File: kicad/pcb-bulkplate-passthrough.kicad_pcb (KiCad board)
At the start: 2 copper layers, 60.8 x 64.2 mm, 9 parts, among them J1 2601-3108

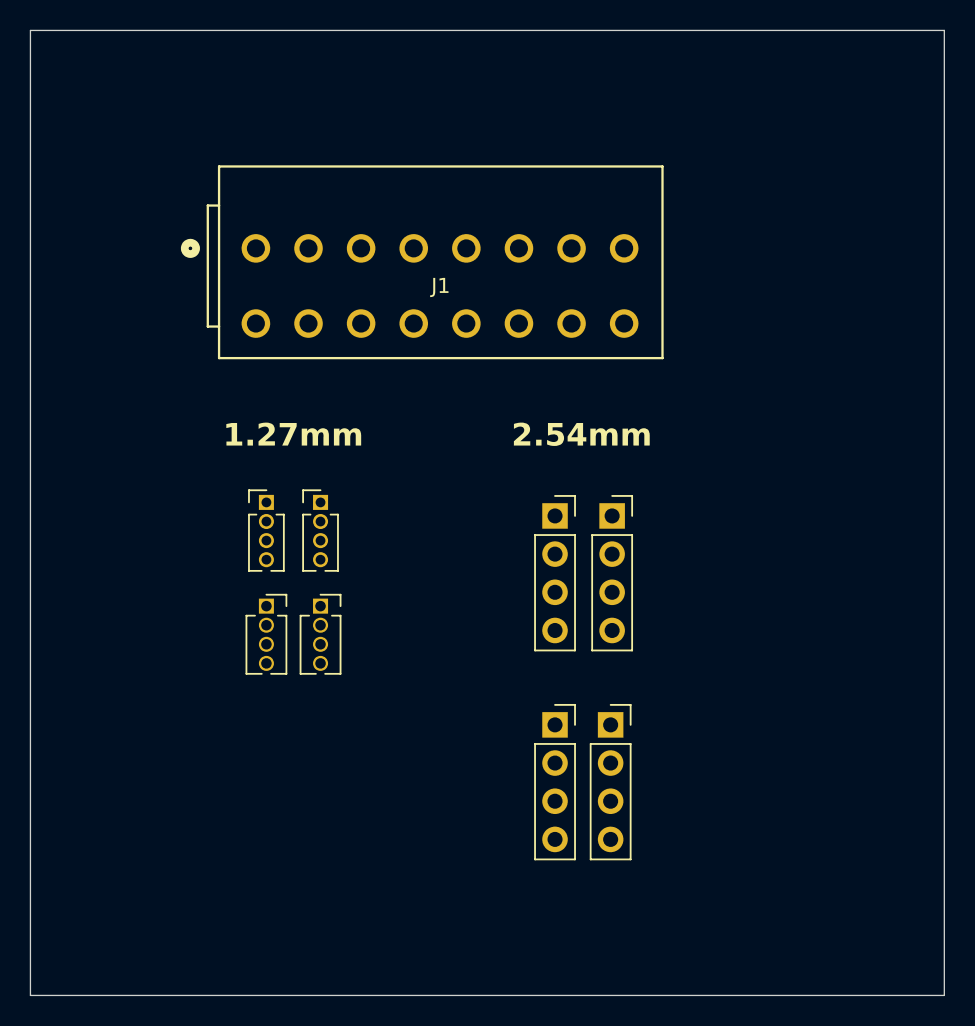
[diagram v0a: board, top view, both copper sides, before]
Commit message: done
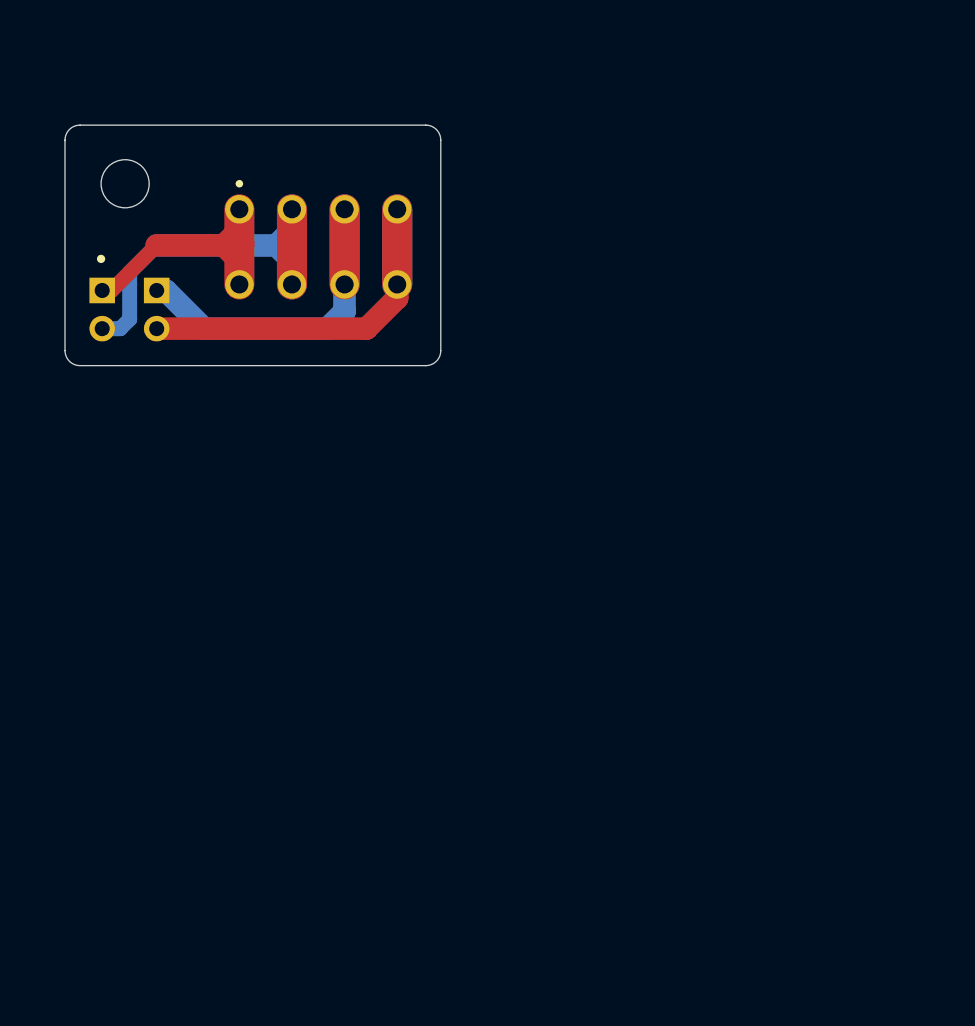
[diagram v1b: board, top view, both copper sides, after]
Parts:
- removed REF** (x2): PinSocket_1x04_P1.27mm_Vertical, Connector_PinSocket_1.27mm:PinSocket_1x04_P1.27mm_Vertical
- removed REF** (x4): PinSocket_1x04_P2.54mm_Vertical, Connector_PinSocket_2.54mm:PinSocket_1x04_P2.54mm_Vertical
- removed REF** (x2): PinHeader_1x04_P1.27mm_Vertical, Connector_PinHeader_1.27mm:PinHeader_1x04_P1.27mm_Vertical
- added H1: M3 Hole, MountingHole:MountingHole_3.2mm_M3, F.Cu at (77.0, 59.9)
- added J2: 2.54mm Header, Connector_PinSocket_2.54mm:PinSocket_1x02_P2.54mm_Vertical, B.Cu at (79.1, 67.0)
- added J3: 2.54mm Header, Connector_PinSocket_2.54mm:PinSocket_1x02_P2.54mm_Vertical, B.Cu at (75.5, 67.0)
- J1: value 2601-3108 -> 2601-3104; footprint 2601-3108:2601-3108 -> 2601-3104:CONN4_2601-3104_WAG
- moved J1 2.82 mm to (84.6, 61.6)
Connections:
- J1 pad 1: unconnected-(J1-Pin_1-Pad1) -> Net-(J1-Pin_1)
- J1 pad 2: unconnected-(J1-Pin_2-Pad2) -> Net-(J1-Pin_2)
- J1 pad 3: unconnected-(J1-Pin_3-Pad3) -> Net-(J1-Pin_3)
- J1 pad 4: unconnected-(J1-Pin_4-Pad4) -> Net-(J1-Pin_4)
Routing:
- net Net-(J1-Pin_2): track 0.00 -> 29.9 mm
- net Net-(J1-Pin_4): track 0.00 -> 27.7 mm
- net Net-(J1-Pin_3): track 0.00 -> 25.8 mm
- net Net-(J1-Pin_1): track 0.00 -> 18.2 mm
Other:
- board size 60.8 x 64.2 mm -> 25 x 16 mm
- board text removed: "1.27mm"
- board text removed: "2.54mm"
